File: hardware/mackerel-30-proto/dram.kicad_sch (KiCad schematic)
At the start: 21 parts, among them J11 Conn_02x05_Odd_Even, U10 SIMM72, U9 EPM7128, X3 CXO_DIP14

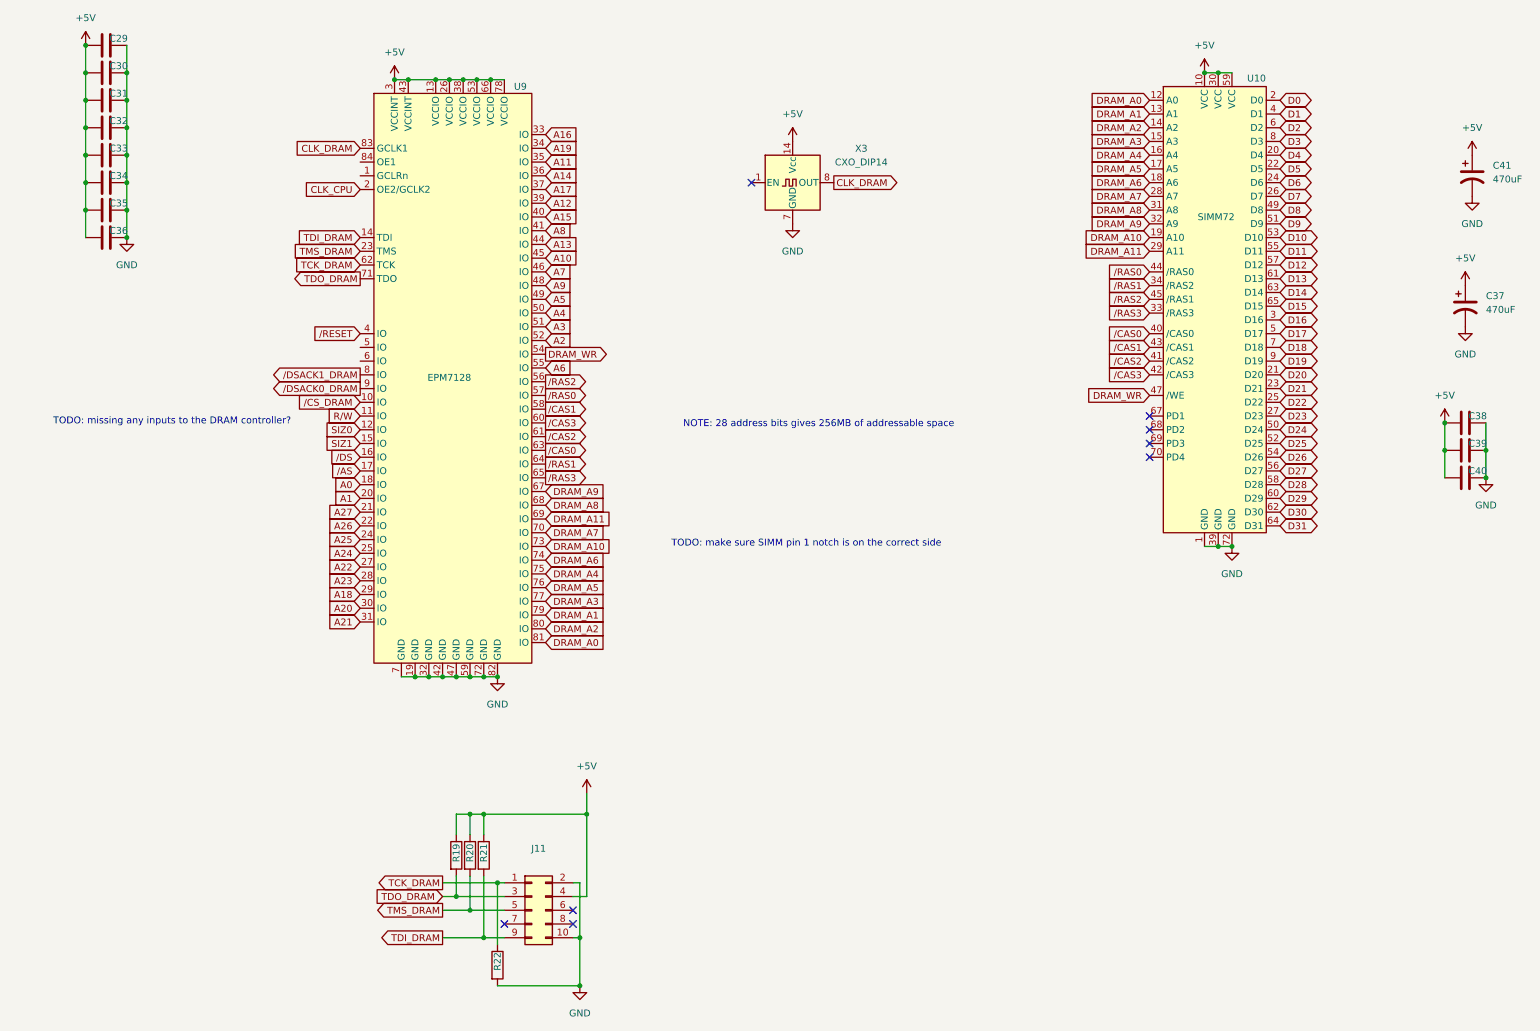
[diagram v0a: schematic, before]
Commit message: PCB cleanup
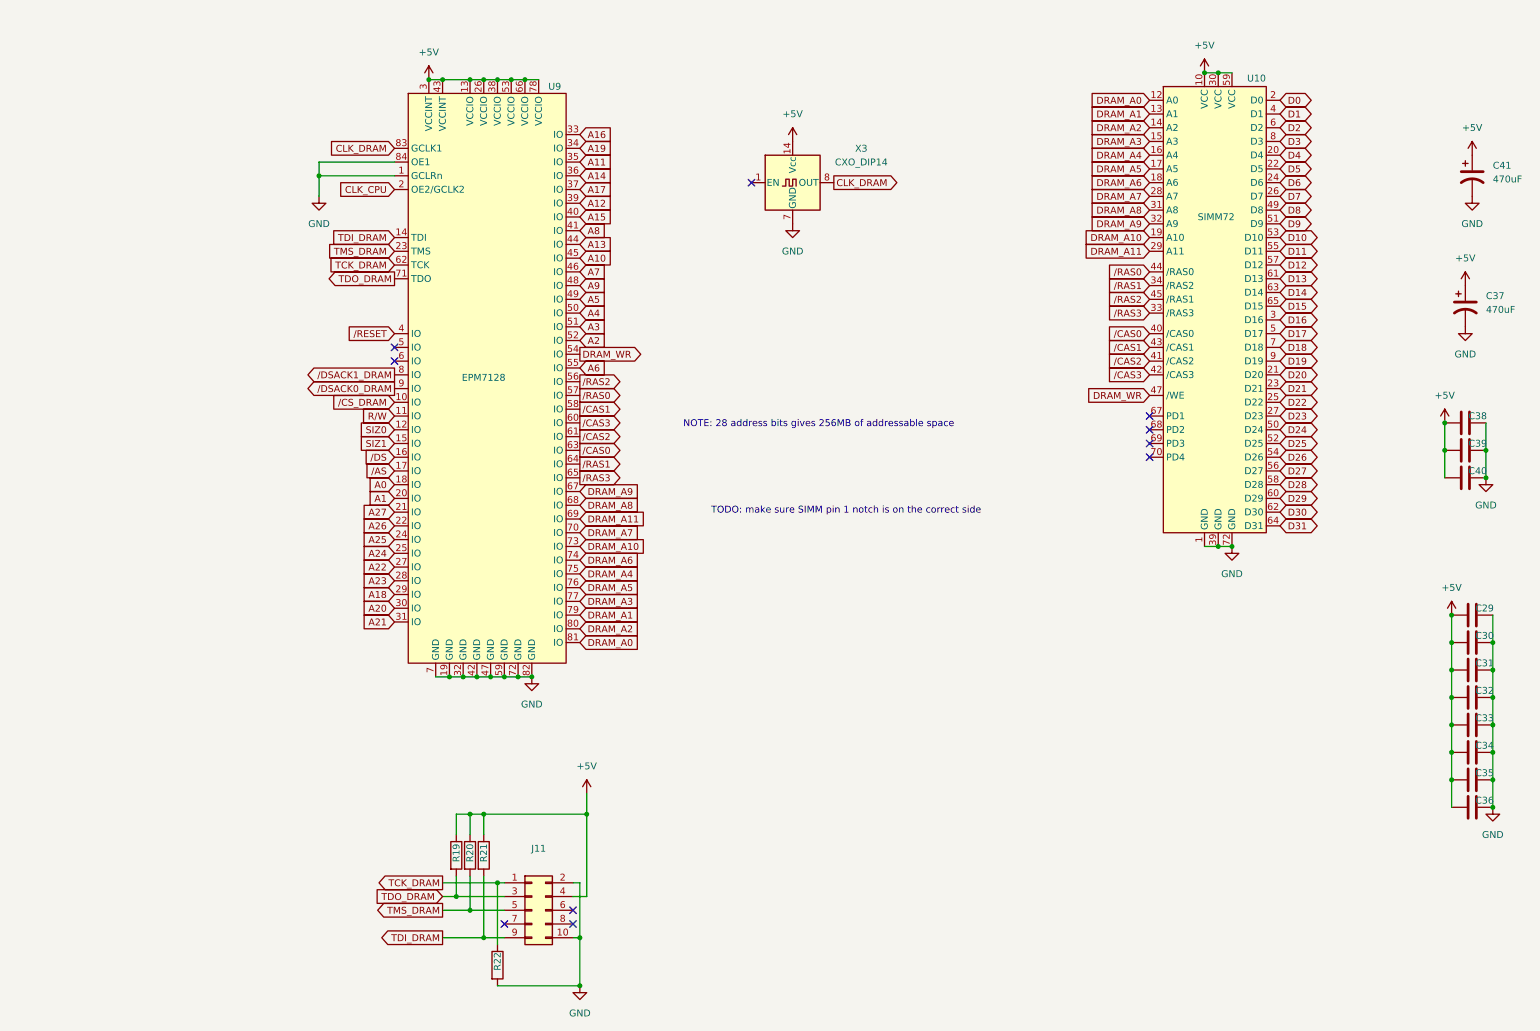
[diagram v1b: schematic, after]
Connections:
- net GND: now also U9.1 (GCLRn), U9.84 (OE1)
- no-connect marks 8 -> 10
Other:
- note removed: "TODO: missing any inputs to the DRAM controller?"
- title: Mackerel-30 Proto -> Mackerel-30
- moved on the sheet: C29, C30, C31, C32, C33, C34, C35, C36, U9
